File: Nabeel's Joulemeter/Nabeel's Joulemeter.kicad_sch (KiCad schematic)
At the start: 26 parts, among them J1 XT60-M, J2 XT60-M, J3 22035035, J4 22035035, U1 INA181A1QDBVRQ1, U2 PADS131M04QPWRQ1, U3 UA78M05QDCYRG4Q1, U4 MCP6286T-E/OT

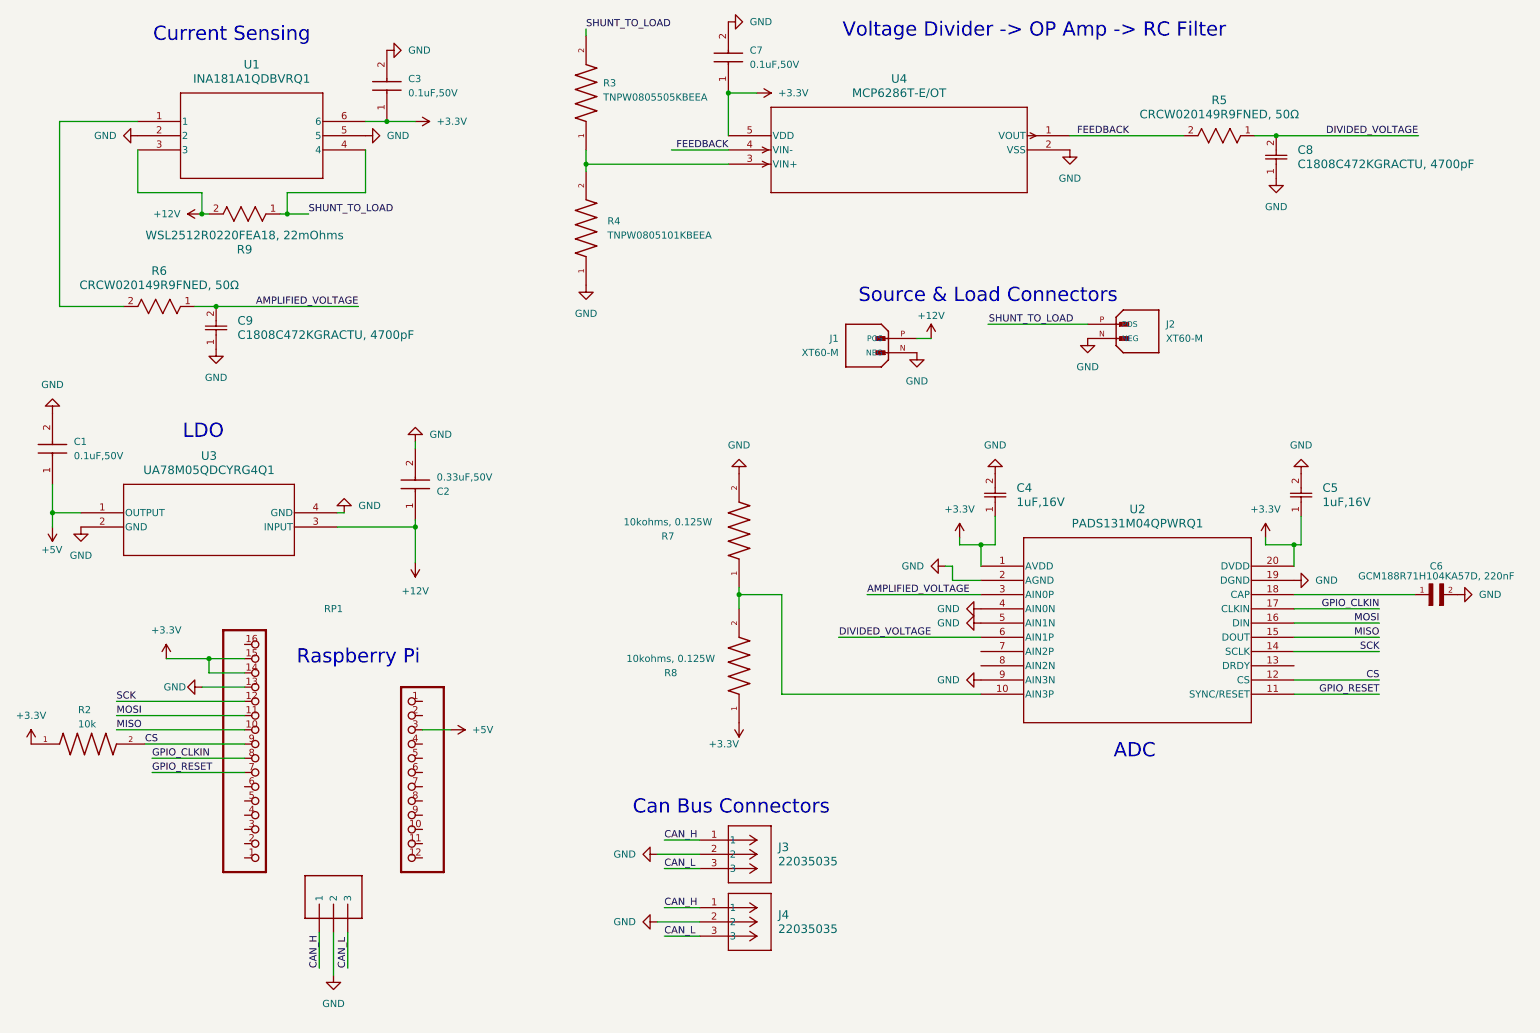
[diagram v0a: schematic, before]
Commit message: RAHHHHH FINISHED MY SCHEMATIC
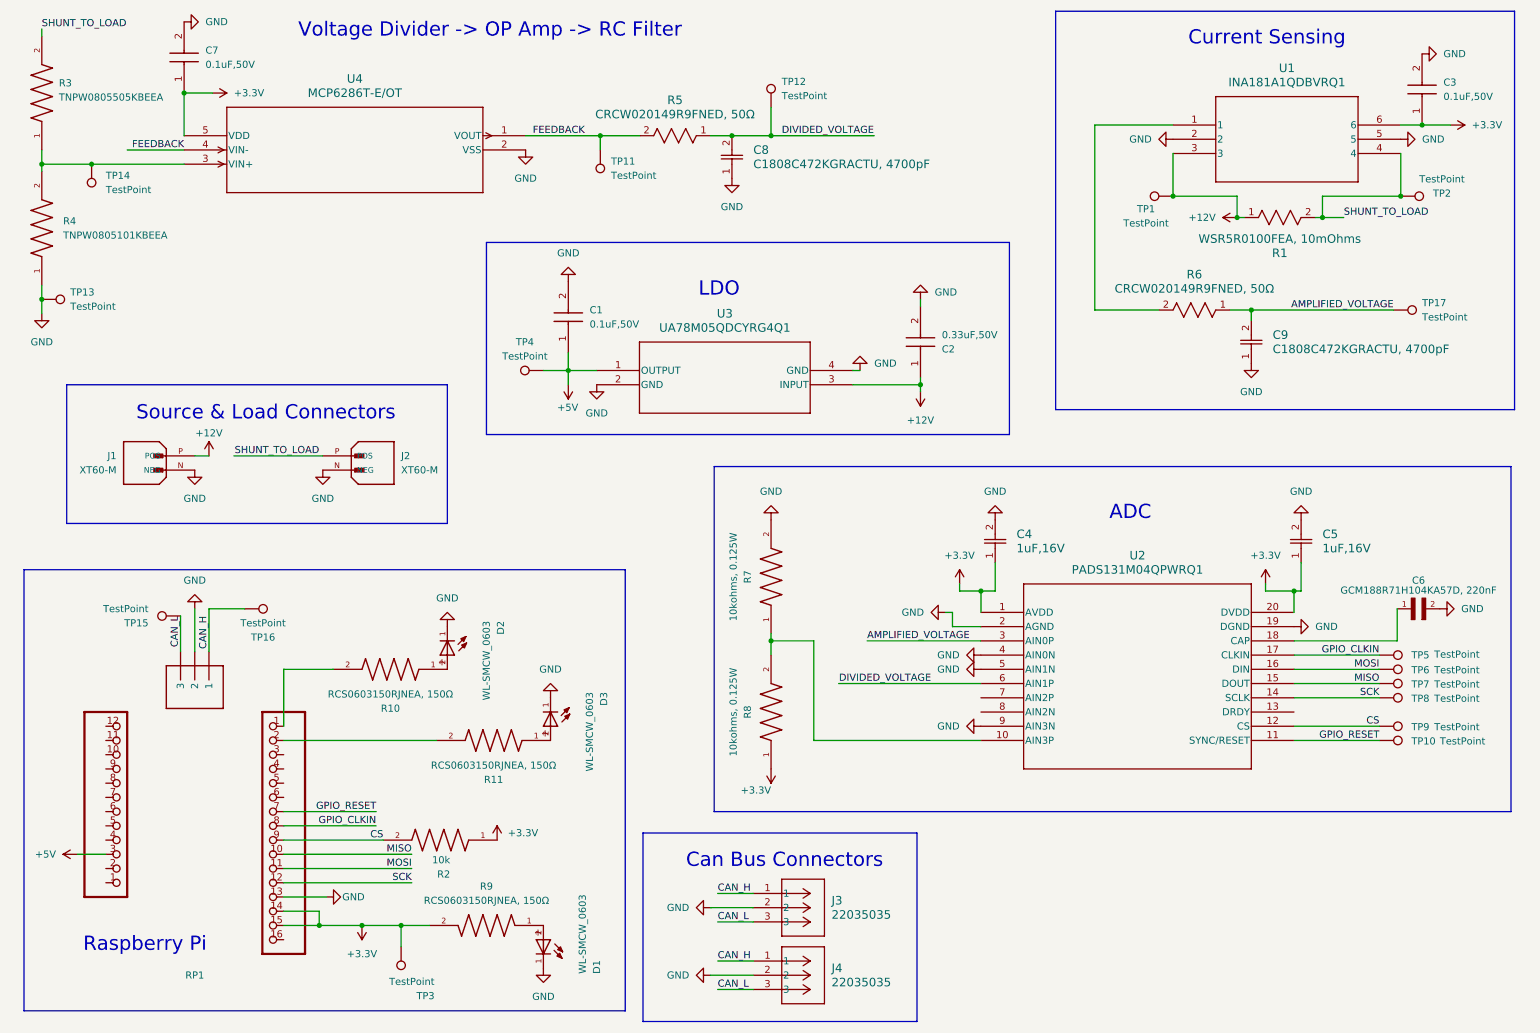
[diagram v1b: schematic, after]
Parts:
- removed R9: WSL2512R0220FEA18, 22mOhms, WSL2512_VIS, symbol SMV_Custom:WSL2512R0220FEA18
- added D1, D2, D3: WL-SMCW_0603, SMV_Passives:WL-SMCW_0603(diode), symbol SMV_Custom:WL-SMCW_0603
- added R1: WSR5R0100FEA, 10mOhms, WSR, symbol SMV_Custom:WSR5R0100FEA
- added R10, R11, R9: RCS0603150RJNEA, 150Ω, SMV_Passives:0805RESC2012X60N, symbol SMV_Custom:RCS0603150RJNEA
- added TP1, TP10, TP11, TP12, TP13, TP14, TP15, TP16, TP17, TP2, TP3, TP4, TP5, TP6, TP7, TP8, TP9: TestPoint, symbol Connector:TestPoint
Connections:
- net +12V: now also R1.1, TP1.1
- net +3.3V: now also R9.2, TP3.1
- net +5V: now also TP4.1
- net AMPLIFIED_VOLTAGE: now also TP17.1
- net CAN_H: now also TP16.1
- net CAN_L: now also TP15.1
- net CS: now also TP9.1
- net DIVIDED_VOLTAGE: now also TP12.1
- net FEEDBACK: now also TP11.1
- net GND: now also D1.1, D2.1, D3.1, TP13.1
- net GPIO_CLKIN: now also TP5.1
- net GPIO_RESET: now also TP10.1
- net MISO: now also TP7.1
- net MOSI: now also TP6.1
- net SCK: now also TP8.1
- net SHUNT_TO_LOAD: now also R1.2, TP2.1
- net at R3.1, R4.2, U4.3 (VIN+): now also TP14.1
- new net: D3.2, R11.1
- new net: R11.2, RP1.2
- new net: D2.2, R10.1
- new net: R10.2, RP1.1
- new net: D1.2, R9.1
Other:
- moved on the sheet: C1, C2, C3, C4, C5, C6, C7, C8, C9, J1, J2, J3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
